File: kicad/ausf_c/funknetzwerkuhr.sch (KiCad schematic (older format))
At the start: 83 parts, among them J4 Conn_01x04_Male, Q10 MMBTA42, Q11 MMBTA42, Q12 MMBTA42, Q13 MMBTA42, Q14 MMBTA42, Q15 MMBTA42, Q16 MMBTA42, Q17 MMBTA42, Q18 MMBTA42, Q19 MMBTA42, Q2 MMBTA42, Q20 MMBTA42, Q21 MMBTA42, Q22 MMBTA42, Q3 MMBTA92, Q4 MMBTA42, Q5 MMBTA92, Q6 MMBTA42, Q7 MMBTA92, Q8 MMBTA42, Q9 MMBTA92, U1 74HC595, U2 74HC595, U3 74HC595, U5 NCP1117-33G, U6 ESP-12E

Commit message: Nearly done Ausf C PCB layout.
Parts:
- Q10, Q11, Q12, Q13, Q14, Q15, Q16, Q17, Q18, Q19, Q2, Q20, Q21, Q22, Q4, Q6, Q8: footprint Package_TO_SOT_SMD:TSOT-23_HandSoldering -> PartsStash:MPSA42-TSOT-23_HandSoldering; symbol Parts_Stash:MMBTA42 -> funknetzwerkuhr-rescue:MMBTA42-Parts_Stash
- Q3, Q5, Q7, Q9: footprint Package_TO_SOT_SMD:TSOT-23_HandSoldering -> PartsStash:MPSA92-TSOT-23_HandSoldering; symbol Parts_Stash:MMBTA92 -> funknetzwerkuhr-rescue:MMBTA92-Parts_Stash
- R10, R11, R12, R13, R14, R15, R16, R17, R18, R19, R20, R21, R22, R23, R24, R25, R26, R27, R28, R29, R3, R30, R31, R32, R33, R35, R36, R37, R39, R4, R40, R41, R42, R43, R44, R45, R46, R47, R48, R49, R5, R6, R7, R8, R9: footprint Resistor_SMD:R_0805_2012Metric_Pad1.15x1.40mm_HandSolder -> PartsStash:R_0805_2012Metric_Pad1.15x1.40mm_HandSolder_Value
- U6: symbol ESP8266:ESP-12E -> funknetzwerkuhr-rescue:ESP-12E-ESP8266
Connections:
- wire segments 221 -> 225
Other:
- moved on the sheet: R37

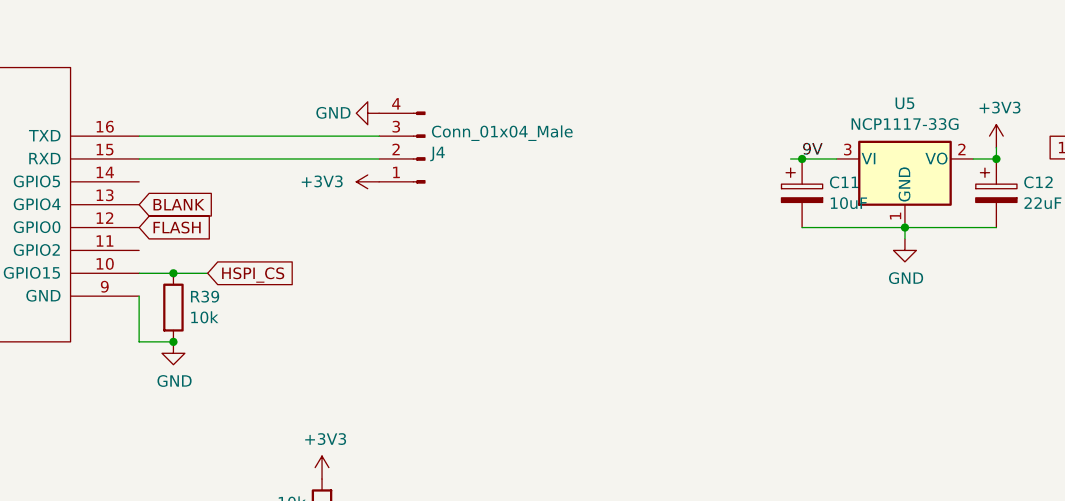
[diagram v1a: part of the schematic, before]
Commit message: Ausf C PCB version ordered.
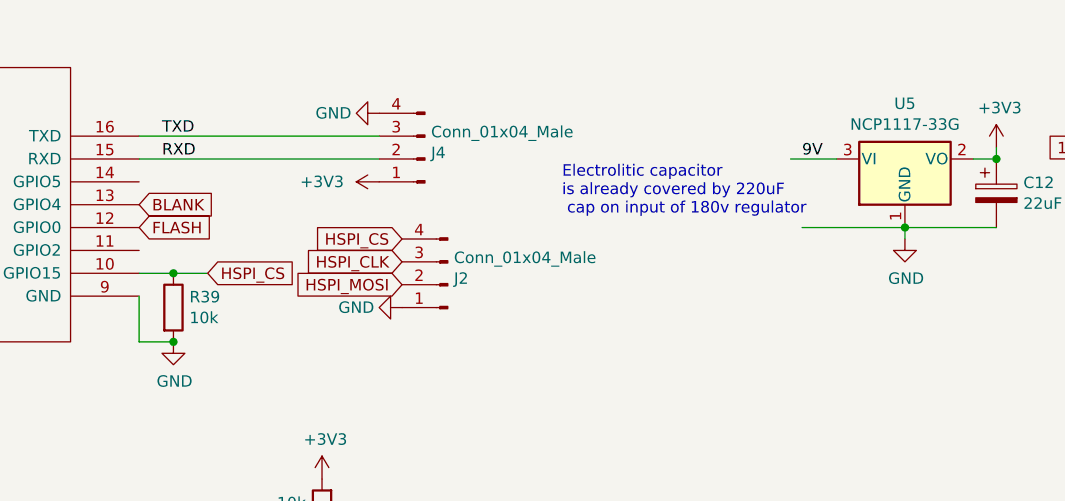
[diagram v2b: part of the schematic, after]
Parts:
- removed C11: 10uF, Capacitor_SMD:CP_Elec_6.3x5.4, symbol Device:CP
- added J2: Conn_01x04_Male, Connector_PinHeader_2.54mm:PinHeader_1x04_P2.54mm_Vertical, symbol Connector:Conn_01x04_Male
- C12: footprint Capacitor_SMD:CP_Elec_6.3x5.4 -> Capacitor_THT:CP_Radial_D6.3mm_P2.50mm
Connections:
- net GND: now also J2.1 (Pin_1)
- net HSPI_CLK: now also J2.3 (Pin_3)
- net HSPI_CS: now also J2.4 (Pin_4)
- net HSPI_MOSI: now also J2.2 (Pin_2)
- net RXD: now reaches J4.2 (Pin_2), U6.15 (RXD)
- net TXD: now reaches J4.3 (Pin_3), U6.16 (TXD)
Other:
- note added: "Electrolitic capacitor \nis already covered by 220uF\n cap on input of 180v regulator"
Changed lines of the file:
@@
 	1    0    0    -1
 $EndComp
-Wire Wire Line
-	6000 950  6050 950
 $Comp
 L power:+3V3 #PWR015
@@
 Connection ~ 6700 3400
 $Comp
-L Device:CP C11
-U 1 1 5B6D84E6
-P 6050 1100
-F 0 "C11" H 6168 1146 50  0000 L CNN
-F 1 "10uF" H 6168 1055 50  0000 L CNN
-F 2 "Capacitor_SMD:CP_Elec_6.3x5.4" H 6088 950 50  0001 C CNN
-F 3 "~" H 6050 1100 50  0001 C CNN
-	1    6050 1100
-	1    0    0    -1
-$EndComp
-Connection ~ 6050 950
-Wire Wire Line
-	6050 950  6200 950
-$Comp
 L Device:CP C12
 U 1 1 5B6D89E2
@@
 F 0 "C12" H 7018 1146 50  0000 L CNN
 F 1 "22uF" H 7018 1055 50  0000 L CNN
-F 2 "Capacitor_SMD:CP_Elec_6.3x5.4" H 6938 950 50  0001 C CNN
+F 2 "Capacitor_THT:CP_Radial_D6.3mm_P2.50mm" H 6938 950 50  0001 C CNN
 F 3 "~" H 6900 1100 50  0001 C CNN
 	1    6900 1100
@@
 	-1   0    0    1
 $EndComp
-Wire Bus Line
-	7650 2850 10000 2850
-Wire Bus Line
-	10000 2850 10000 3400
-Wire Bus Line
-	750  6400 11150 6400
-Wire Bus Line
-	700  4500 11150 4500
-Wire Bus Line
-	10000 600  10000 2850
 $Comp
 L funknetzwerkuhr-rescue:MMBTA42-Parts_Stash Q13
@@
 	1    0    0    1
 $EndComp
+Wire Wire Line
+	6000 950  6200 950
+Text Notes 5000 1200 0    50   ~ 0
+Electrolitic capacitor \nis already covered by 220uF\n cap on input of 180v regulator
+Text Label 3250 850  0    50   ~ 0
+TXD
+Text Label 3250 950  0    50   ~ 0
+RXD
+$Comp
+L Connector:Conn_01x04_Male J2
+U 1 1 5CE3FFDC
+P 4500 1500
+F 0 "J2" H 4473 1473 50  0000 R CNN
+F 1 "Conn_01x04_Male" H 4473 1382 50  0000 R CNN
+F 2 "Connector_PinHeader_2.54mm:PinHeader_1x04_P2.54mm_Vertical" H 4500 1500 50  0001 C CNN
+F 3 "~" H 4500 1500 50  0001 C CNN
+	1    4500 1500
+	-1   0    0    1
+$EndComp
+Text GLabel 4300 1300 0    50   Input ~ 0
+HSPI_CS
+Text GLabel 4300 1400 0    50   Input ~ 0
+HSPI_CLK
+Text GLabel 4300 1500 0    50   Input ~ 0
+HSPI_MOSI
+$Comp
+L power:GND #PWR049
+U 1 1 5CE41997
+P 4300 1600
+F 0 "#PWR049" H 4300 1350 50  0001 C CNN
+F 1 "GND" V 4300 1400 50  0000 C CNN
+F 2 "" H 4300 1600 50  0001 C CNN
+F 3 "" H 4300 1600 50  0001 C CNN
+	1    4300 1600
+	0    1    1    0
+$EndComp
+Wire Bus Line
+	7650 2850 10000 2850
+Wire Bus Line
+	10000 2850 10000 3400
+Wire Bus Line
+	10000 600  10000 2850
+Wire Bus Line
+	750  6400 11150 6400
+Wire Bus Line
+	700  4500 11150 4500
 $EndSCHEMATC

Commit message: Opened ausf_c with newer Kicad version.
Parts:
- Q10, Q11, Q12, Q13, Q14, Q15, Q16, Q17, Q18, Q19, Q2, Q20, Q21, Q22, Q4, Q6, Q8: symbol funknetzwerkuhr-rescue:MMBTA42-Parts_Stash -> funknetzwerkuhr-rescue:MMBTA42-Parts_Stash-funknetzwerkuhr-rescue
- Q3, Q5, Q7, Q9: symbol funknetzwerkuhr-rescue:MMBTA92-Parts_Stash -> funknetzwerkuhr-rescue:MMBTA92-Parts_Stash-funknetzwerkuhr-rescue
- U6: symbol funknetzwerkuhr-rescue:ESP-12E-ESP8266 -> funknetzwerkuhr-rescue:ESP-12E-ESP8266-funknetzwerkuhr-rescue
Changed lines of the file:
@@
 EESchema Schematic File Version 4
-LIBS:funknetzwerkuhr-cache
-EELAYER 29 0
+EELAYER 30 0
 EELAYER END
 $Descr A4 11693 8268
@@
 $EndSheet
 $Comp
-L funknetzwerkuhr-rescue:MMBTA92-Parts_Stash Q?
+L funknetzwerkuhr-rescue:MMBTA92-Parts_Stash-funknetzwerkuhr-rescue Q?
 U 1 1 5B5C06CE
 P 1350 5150
@@
 	1450 6300 1450 5750
 $Comp
-L funknetzwerkuhr-rescue:MMBTA42-Parts_Stash Q?
+L funknetzwerkuhr-rescue:MMBTA42-Parts_Stash-funknetzwerkuhr-rescue Q?
 U 1 1 5B5C06D9
 P 1050 5850
@@
 	10000 900  10100 1000
 $Comp
-L funknetzwerkuhr-rescue:MMBTA92-Parts_Stash Q?
+L funknetzwerkuhr-rescue:MMBTA92-Parts_Stash-funknetzwerkuhr-rescue Q?
 U 1 1 5B6151F7
 P 2250 5150
@@
 	2350 6300 2350 5750
 $Comp
-L funknetzwerkuhr-rescue:MMBTA42-Parts_Stash Q?
+L funknetzwerkuhr-rescue:MMBTA42-Parts_Stash-funknetzwerkuhr-rescue Q?
 U 1 1 5B615200
 P 1950 5850
@@
 DRIVE_BLUE
 $Comp
-L funknetzwerkuhr-rescue:MMBTA92-Parts_Stash Q?
+L funknetzwerkuhr-rescue:MMBTA92-Parts_Stash-funknetzwerkuhr-rescue Q?
 U 1 1 5B61DCAA
 P 3150 5150
@@
 	3250 6300 3250 5750
 $Comp
-L funknetzwerkuhr-rescue:MMBTA42-Parts_Stash Q?
+L funknetzwerkuhr-rescue:MMBTA42-Parts_Stash-funknetzwerkuhr-rescue Q?
 U 1 1 5B61DCB3
 P 2850 5850
@@
 	2350 5450 2350 5350
 $Comp
-L funknetzwerkuhr-rescue:MMBTA92-Parts_Stash Q?
+L funknetzwerkuhr-rescue:MMBTA92-Parts_Stash-funknetzwerkuhr-rescue Q?
 U 1 1 5B657A9D
 P 4050 5150
@@
 	4150 6300 4150 5750
 $Comp
-L funknetzwerkuhr-rescue:MMBTA42-Parts_Stash Q?
+L funknetzwerkuhr-rescue:MMBTA42-Parts_Stash-funknetzwerkuhr-rescue Q?
 U 1 1 5B657AA6
 P 3750 5850
@@
 DRIVE_D2
 $Comp
-L funknetzwerkuhr-rescue:MMBTA42-Parts_Stash Q10
+L funknetzwerkuhr-rescue:MMBTA42-Parts_Stash-funknetzwerkuhr-rescue Q10
 U 1 1 5B66EB7A
 P 4600 5150
@@
 	4700 6300 4800 6400
 $Comp
-L funknetzwerkuhr-rescue:MMBTA42-Parts_Stash Q11
+L funknetzwerkuhr-rescue:MMBTA42-Parts_Stash-funknetzwerkuhr-rescue Q11
 U 1 1 5B68C6FD
 P 5150 5150
@@
 	5250 6300 5350 6400
 $Comp
-L funknetzwerkuhr-rescue:MMBTA42-Parts_Stash Q12
+L funknetzwerkuhr-rescue:MMBTA42-Parts_Stash-funknetzwerkuhr-rescue Q12
 U 1 1 5B68F8EA
 P 5650 5150
@@
 	6250 6300 6350 6400
 $Comp
-L funknetzwerkuhr-rescue:MMBTA42-Parts_Stash Q14
+L funknetzwerkuhr-rescue:MMBTA42-Parts_Stash-funknetzwerkuhr-rescue Q14
 U 1 1 5B6968F8
 P 6650 5150
@@
 	6750 6300 6850 6400
 $Comp
-L funknetzwerkuhr-rescue:MMBTA42-Parts_Stash Q15
+L funknetzwerkuhr-rescue:MMBTA42-Parts_Stash-funknetzwerkuhr-rescue Q15
 U 1 1 5B69A76F
 P 7150 5150
@@
 	7250 6300 7350 6400
 $Comp
-L funknetzwerkuhr-rescue:MMBTA42-Parts_Stash Q16
+L funknetzwerkuhr-rescue:MMBTA42-Parts_Stash-funknetzwerkuhr-rescue Q16
 U 1 1 5B69E9E7
 P 7650 5150
@@
 	7750 6300 7850 6400
 $Comp
-L funknetzwerkuhr-rescue:MMBTA42-Parts_Stash Q17
+L funknetzwerkuhr-rescue:MMBTA42-Parts_Stash-funknetzwerkuhr-rescue Q17
 U 1 1 5B6A3147
 P 8150 5150
@@
 	8250 6300 8350 6400
 $Comp
-L funknetzwerkuhr-rescue:MMBTA42-Parts_Stash Q18
+L funknetzwerkuhr-rescue:MMBTA42-Parts_Stash-funknetzwerkuhr-rescue Q18
 U 1 1 5B6A7F16
 P 8650 5150
@@
 	8750 6300 8850 6400
 $Comp
-L funknetzwerkuhr-rescue:MMBTA42-Parts_Stash Q19
+L funknetzwerkuhr-rescue:MMBTA42-Parts_Stash-funknetzwerkuhr-rescue Q19
 U 1 1 5B6ACF8A
 P 9150 5150
@@
 	9250 6300 9350 6400
 $Comp
-L funknetzwerkuhr-rescue:MMBTA42-Parts_Stash Q20
+L funknetzwerkuhr-rescue:MMBTA42-Parts_Stash-funknetzwerkuhr-rescue Q20
 U 1 1 5B6B2485
 P 9650 5150
@@
 DOT
 $Comp
-L funknetzwerkuhr-rescue:ESP-12E-ESP8266 U6
+L funknetzwerkuhr-rescue:ESP-12E-ESP8266-funknetzwerkuhr-rescue U6
 U 1 1 5B6C570B
 P 2250 1150
@@
 	10450 4500 10550 4600
 $Comp
-L funknetzwerkuhr-rescue:MMBTA42-Parts_Stash Q22
+L funknetzwerkuhr-rescue:MMBTA42-Parts_Stash-funknetzwerkuhr-rescue Q22
 U 1 1 5B7684A7
 P 10750 5150
@@
 	4150 7050 4150 7100
 $Comp
-L funknetzwerkuhr-rescue:MMBTA42-Parts_Stash Q21
+L funknetzwerkuhr-rescue:MMBTA42-Parts_Stash-funknetzwerkuhr-rescue Q21
 U 1 1 5B6C98E5
 P 10200 5150
@@
 $EndComp
 $Comp
-L funknetzwerkuhr-rescue:MMBTA42-Parts_Stash Q13
+L funknetzwerkuhr-rescue:MMBTA42-Parts_Stash-funknetzwerkuhr-rescue Q13
 U 1 1 5B692F19
 P 6150 5150
